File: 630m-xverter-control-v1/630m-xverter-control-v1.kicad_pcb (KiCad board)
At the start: 2 copper layers, 126.4 x 69.8 mm, 53 parts, among them J1 Rig Transverter, J2 ALC, J3 ANT, J4 TX_TO_AMP, J5 TX_FROM_AMP, J6 Power, J7 TX AMP POWER, K1 DS1E-M-DC12V, K2 DS1E-M-DC12V, K3 DS1E-M-DC12V, Q1 2N3904, Q2 2N3904, Q3 2N3904, Q4 2N3904, Q5 2N3904, Q6 2N3904, Q7 TIP125

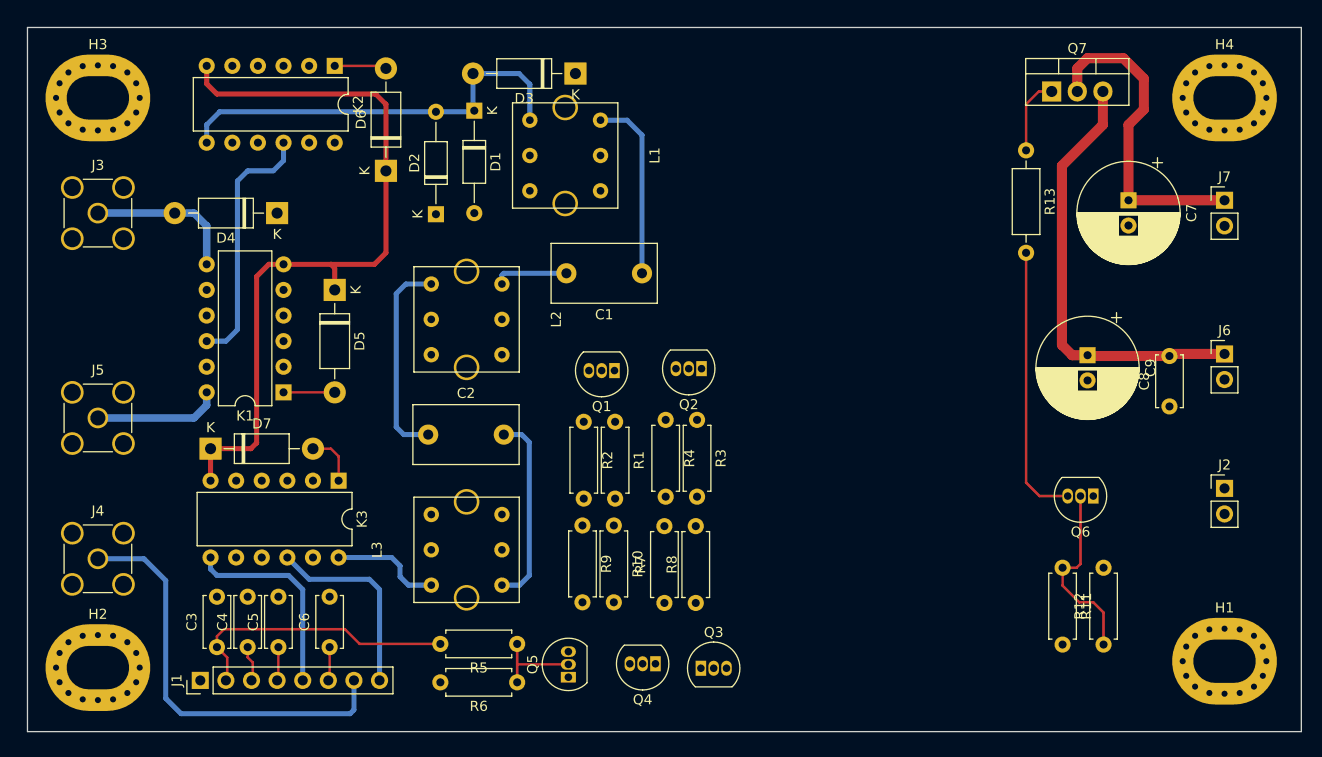
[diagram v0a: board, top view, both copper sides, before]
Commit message: Update PCB layout, it should work? kinda? we'll see.
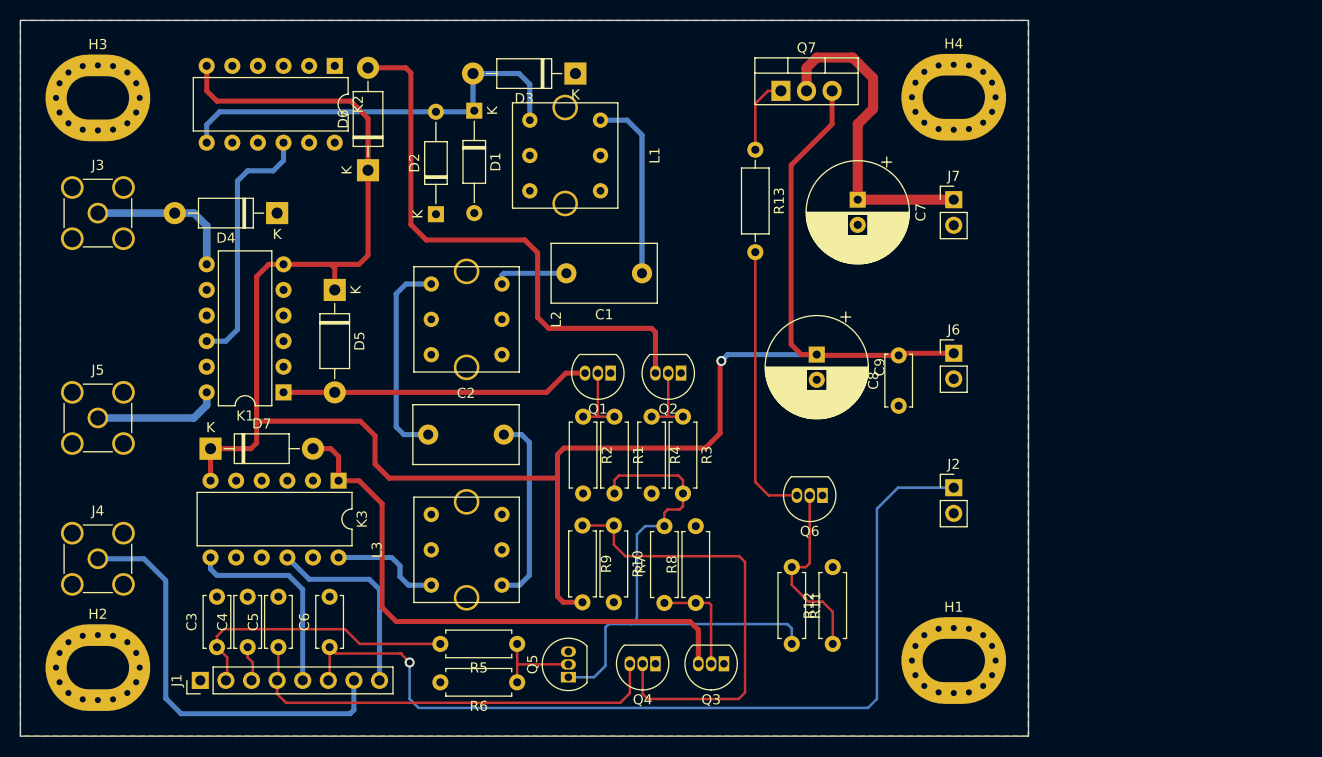
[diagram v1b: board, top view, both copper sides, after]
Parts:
- moved C7 26.9 mm to (95.1, 29.8)
- moved Q6 26.9 mm to (91.6, 59.1)
- moved Q7 26.9 mm to (87.4, 19.0)
- moved R12 26.9 mm to (92.6, 73.9)
- moved R13 26.9 mm to (84.9, 24.8)
- moved C8 26.9 mm to (99.1, 50.2)
- moved C9 26.9 mm to (91.0, 45.1)
- moved H1 26.9 mm to (104.6, 75.5)
- moved H4 26.9 mm to (104.6, 19.6)
- moved J2 26.9 mm to (104.6, 58.4)
- moved J6 26.9 mm to (104.6, 45.0)
- moved J7 26.9 mm to (104.6, 29.8)
- moved R11 26.9 mm to (88.5, 66.2)
- moved Q3 2.33 mm to (81.8, 75.8), turned to 180 degrees
- moved Q2 2.08 mm to (77.5, 47.0)
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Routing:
- net XVERTER_ALC_INPUT: track 3.35 -> 90.1 mm, vias 0 -> 1
- net PA_DISABLE: track 119.6 -> 200.1 mm, vias 0 -> 1
- net TX_ENABLE: track 0.00 -> 55.0 mm
- net Net-(D7-Pad2): track 5.27 -> 56.5 mm
- net Net-(D6-Pad2): track 5.19 -> 56.0 mm
- net Net-(Q4-Pad2): track 0.00 -> 45.3 mm
- net XVERTER_TX_PA_DISABLE: track 3.35 -> 43.4 mm
- net Net-(D5-Pad2): track 5.08 -> 30.7 mm
- net Net-(Q3-Pad2): track 0.00 -> 10.6 mm
- net Net-(Q2-Pad2): track 0.00 -> 7.48 mm
- net Net-(Q1-Pad2): track 0.00 -> 7.43 mm
- added copper zone on B.Cu, net GND
- added copper zone on F.Cu, net GND
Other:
- board size 126.4 x 69.8 mm -> 100 x 71 mm
